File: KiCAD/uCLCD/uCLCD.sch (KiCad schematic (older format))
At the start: 15 parts, among them IC1 ATMEGA328P-P, P1 CONN_01X12, P2 CONN_01X03, P3 CONN_01X02, P4 CONN_01X03, SW1 SW_Push, SW2 SW_Push, SW3 SW_Push, Y1 16Mhz

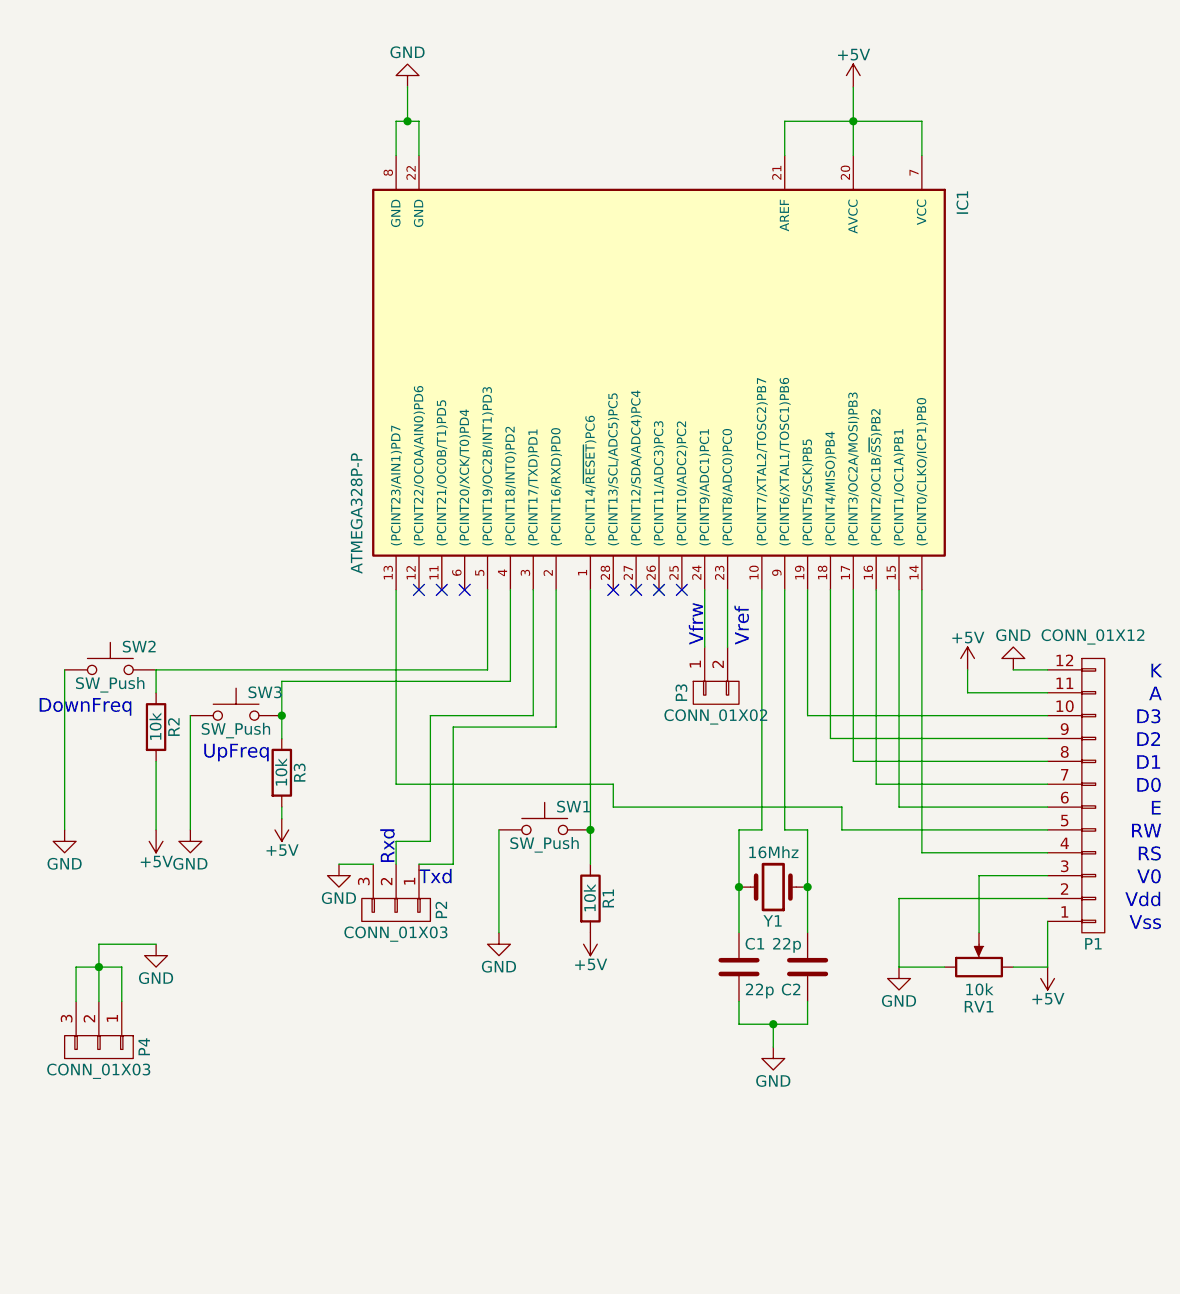
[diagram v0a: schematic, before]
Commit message: Circuit Schematic fixes
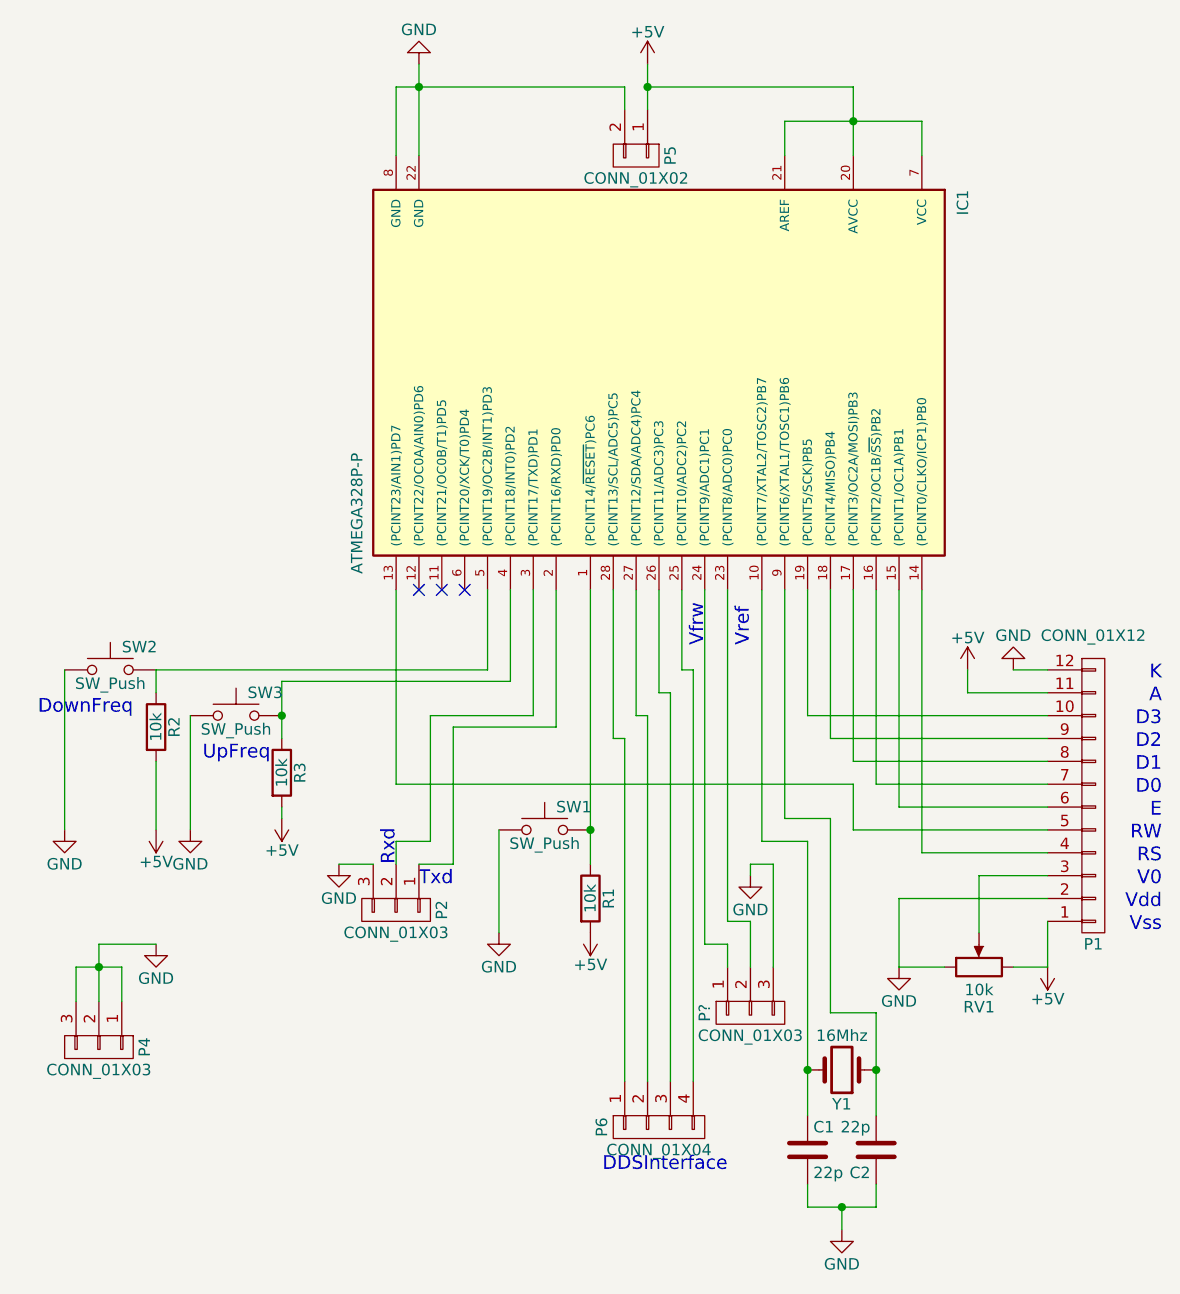
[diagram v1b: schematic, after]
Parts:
- removed P3: CONN_01X02, Pin_Headers:Pin_Header_Straight_1x02, symbol CONN_01X02
- added P5: CONN_01X02, Pin_Headers:Pin_Header_Straight_1x02, symbol CONN_01X02
- added P6: CONN_01X04, Pin_Headers:Pin_Header_Straight_1x04, symbol CONN_01X04
- added P?: CONN_01X03, symbol CONN_01X03
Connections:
- net +5V: now also P5.1 (P1)
- net GND: now also P5.2 (P2), P?.3 (P3)
- net at IC1.23 ((PCINT8/ADC0)PC0): now also P?.2 (P2)
- net at IC1.24 ((PCINT9/ADC1)PC1): now also P?.1 (P1)
- net at IC1.25 ((PCINT10/ADC2)PC2): now also P6.4 (P4)
- net at IC1.26 ((PCINT11/ADC3)PC3): now also P6.3 (P3)
- net at IC1.27 ((PCINT12/SDA/ADC4)PC4): now also P6.2 (P2)
- net at IC1.28 ((PCINT13/SCL/ADC5)PC5): now also P6.1 (P1)
- no-connect marks 7 -> 3
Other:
- note added: "DDSInterface"
- moved on the sheet: C1, C2, Y1
